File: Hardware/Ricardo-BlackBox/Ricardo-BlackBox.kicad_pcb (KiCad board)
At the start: 4 copper layers, 80.3 x 54.1 mm, 87 parts, among them IC1 XTSD08GLGEAG, IC2 CP2102N-A02-GQFN24, J1 RBUS, J2 USB_C_Receptacle_USB2.0, U1 ESP32-S3, U2 SN65HVD230, U3 LM66200DRLR, U4 MAX77827AEFD+T, U5 SC4215, Y1 40MHz±10ppm

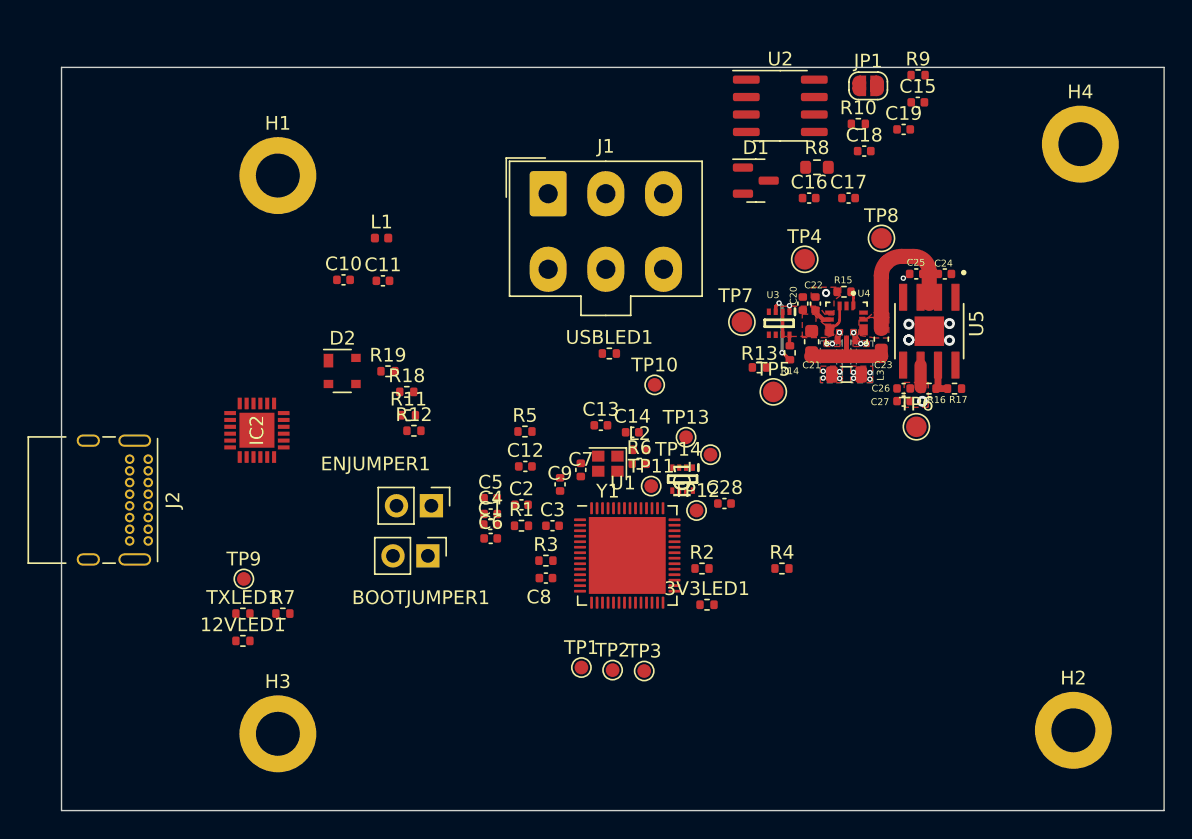
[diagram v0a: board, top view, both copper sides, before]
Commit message: Initial hardware update
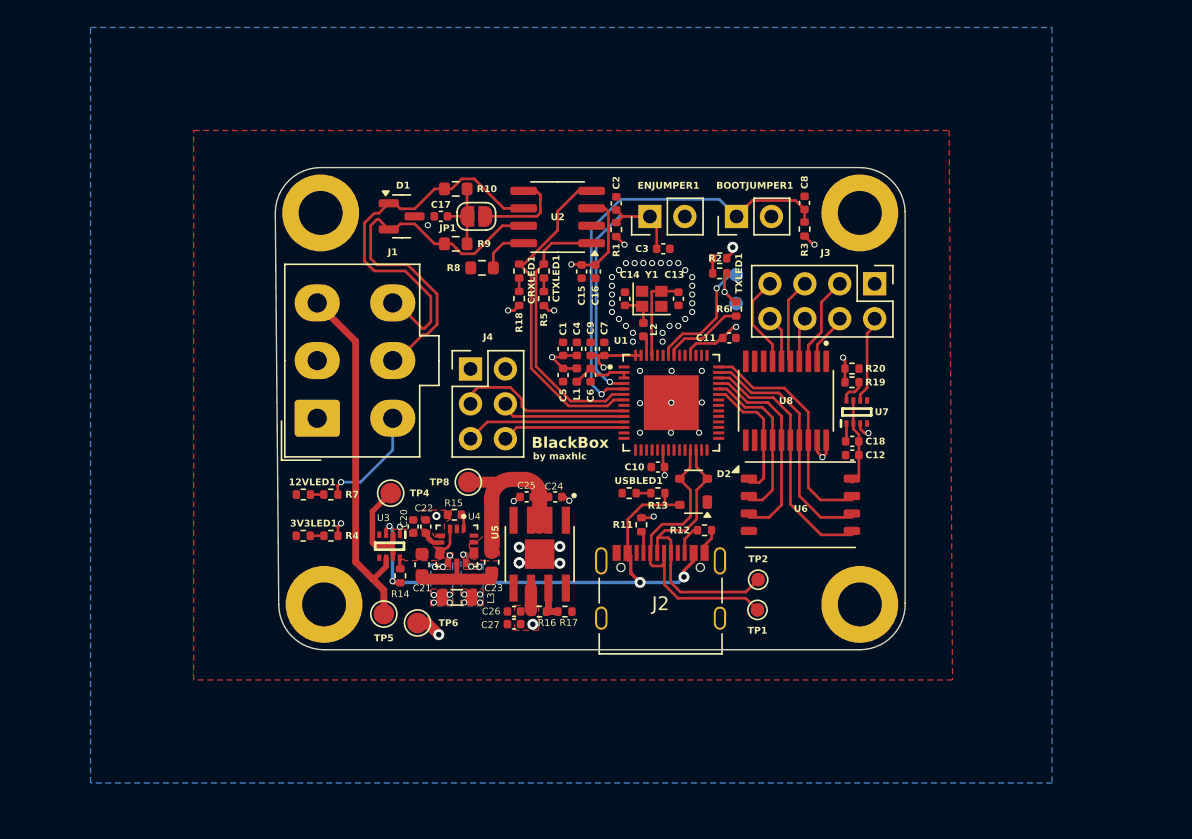
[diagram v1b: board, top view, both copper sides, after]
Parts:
- removed C19: 220pF, Capacitor_SMD:C_0402_1005Metric
- removed C28: 10uF, Capacitor_SMD:C_0402_1005Metric
- removed IC1: XTSD08GLGEAG, iclr:SOTFL50P160X60-8N
- removed IC2: CP2102N-A02-GQFN24, iclr:QFN50P400X400X80-25N
- removed TP11, TP12, TP13, TP14, TP3: TestPoint, TestPoint:TestPoint_Pad_D1.0mm
- removed TP7: TestPoint, TestPoint:TestPoint_Pad_D1.5mm
- added CRXLED1: ORANGE_LED, Resistor_SMD:R_0402_1005Metric, F.Cu at (97.1, 53.3)
- added CTXLED1: GREEN_LED, Resistor_SMD:R_0402_1005Metric, F.Cu at (98.9, 53.3)
- added J3: Conn_02x04_Odd_Even, Connector_PinHeader_2.54mm:PinHeader_2x04_P2.54mm_Vertical, F.Cu at (123.0, 54.2)
- added J4: Conn_02x03_Odd_Even, Connector_PinHeader_2.54mm:PinHeader_2x03_P2.54mm_Vertical, F.Cu at (93.6, 60.5)
- added R20: 10K, Resistor_SMD:R_0402_1005Metric, F.Cu at (121.4, 60.4)
- added U6: XTSD08G, Package_LGA:LGA-8_8x6mm_P1.27mm, F.Cu at (117.6, 70.3)
- added U7: LM66200DRLR, iclr:SOTFL50P160X60-8N, F.Cu at (121.7, 63.6)
- added U8: SN74CBTLV3245APWR, SN74CBTLV3245APWR:SOP65P640X120-20N, F.Cu at (116.5, 62.8)
- 12VLED1: value 12V_LED -> RED_LED
- 3V3LED1: value 3V3LED -> BLUE_LED
- C12: value 4.2pF -> 10uF
- C13, C14: value C -> 11pF
- C17: value 0.1uF -> 47nF
- C18: value 220pF -> 0.1uF
- J2: footprint Connector_USB:USB_C_Receptacle_GCT_USB4085 -> Connector_USB:USB_C_Receptacle_Palconn_UTC16-G
- R10, R9: footprint Resistor_SMD:R_0402_1005Metric -> Resistor_SMD:R_0603_1608Metric
- R13: value 470 -> 5.1k
- R18: value 22.1k -> 1k
- R19: value 47.5k -> 10K
- R5: value 47.5 -> 1k
- R6: value 499 -> 499R
- TP10, TP9: moved to B.Cu
- TXLED1: value TX_LED -> GREEN_LED
- U1: footprint Package_DFN_QFN:QFN-56-1EP_7x7mm_P0.4mm_EP5.6x5.6mm -> iclr:QFN40P700X700X90-57N
- U5: value SC4215 -> SC4215ASTRT
- USBLED1: value USB_LED -> WHITE_LED
- Y1: value 40MHz±10ppm -> R940000171
- moved H4 64.4 mm to (82.9, 77.6)
- moved H3 43.4 mm to (121.9, 77.6)
- moved TXLED1 42.6 mm to (111.7, 53.5), turned to 180 degrees
- moved TP9 41.1 mm to (112.9, 55.7), turned to 180 degrees
- moved H2 40.7 mm to (121.9, 49.1)
- moved TP6 39.0 mm to (89.7, 78.9)
- moved J2 38.5 mm to (107.4, 76.3), turned to 0 degrees
- moved R9 35.8 mm to (92.5, 51.3)
- moved TP8 34.9 mm to (93.4, 68.7)
- moved TP4 34.6 mm to (87.8, 69.5)
- moved R19 33.8 mm to (121.4, 61.4), turned to 180 degrees
- moved BOOTJUMPER1 33.4 mm to (113.0, 49.4), turned to 90 degrees
- moved C8 33.2 mm to (117.9, 48.4), turned to 90 degrees
- moved R4 32.9 mm to (83.4, 72.6)
- moved C21 32.7 mm to (90.1, 74.7)
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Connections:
- C12 pad 1: Net-(C12-Pad1) -> /NAND_3V3
- C12 pad 2: Net-(C12-Pad2) -> GND
- C18 pad 1: GND -> /NAND_3V3
- C18 pad 2: /CAN+ -> GND
- D2 pad 2: Net-(D2-Pad2) -> /Data+
- D2 pad 3: Net-(D2-Pad3) -> /Data-
- D2 pad 4: Net-(D2-Pad4) -> VBUS
- J2 pad A4: Net-(D2-Pad2) -> VBUS
- J2 pad A6: Net-(D2-Pad3) -> /Data+
- J2 pad A7: Net-(D2-Pad4) -> /Data-
- J2 pad A9: Net-(D2-Pad2) -> VBUS
- J2 pad B4: Net-(D2-Pad2) -> VBUS
- J2 pad B6: Net-(D2-Pad3) -> /Data+
- J2 pad B7: Net-(D2-Pad4) -> /Data-
- J2 pad B9: Net-(D2-Pad2) -> VBUS
- R18 pad 1: Net-(D2-Pad2) -> +3V3
- R18 pad 2: Net-(IC2-Pad8) -> Net-(CRXLED1-A)
- R19 pad 1: Net-(IC2-Pad8) -> Net-(U7-ST)
- R19 pad 2: GND -> +3V3
- R5 pad 1: GND -> +3V3
- R5 pad 2: Net-(C12-Pad1) -> Net-(CTXLED1-A)
- R6 pad 1: /RXD -> /TXD
- U1 pad 1: Net-(C12-Pad2) -> unconnected-(U1-LNA_IN/RF-Pad1)
- U1 pad 10: unconnected-(U1-Pad10) -> /GPIO_5
- U1 pad 11: unconnected-(U1-Pad11) -> /GPIO_6
- U1 pad 12: unconnected-(U1-Pad12) -> /GPIO_7
- U1 pad 37: unconnected-(U1-Pad37) -> /NAND_SD2
- U1 pad 38: unconnected-(U1-Pad38) -> /NAND_SD3
- U1 pad 39: unconnected-(U1-Pad39) -> /NAND_CLK
- U1 pad 40: /NAND_CS -> /NAND_CMD
- U1 pad 41: /CLK -> /NAND_SD0
- U1 pad 42: /MISO -> /NAND_SD1
- U1 pad 43: /MOSI -> unconnected-(U1-GPIO38-Pad43)
- U1 pad 50: /TXD -> /RXD
- U1 pad 6: unconnected-(U1-Pad6) -> /CAN_TX
- U1 pad 7: unconnected-(U1-Pad7) -> /CAN_RX
- U1 pad 9: unconnected-(U1-Pad9) -> /GPIO_4
- U5 pad 5: (no net) -> unconnected-(U5-NC-Pad5)
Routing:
- net +3V3: track 1.61 -> 37.6 mm, vias 1 -> 16
- net VBUS: track 5.27 -> 39.7 mm, vias 2 -> 4
- net /BOOT: track 0.00 -> 32.8 mm, vias 0 -> 1
- net /CAN+: track 0.00 -> 30.0 mm
- net /CAN-: track 0.00 -> 29.8 mm
- net RBUS_uC_V: track 0.00 -> 26.3 mm
- net /CAN_RX: track 0.00 -> 24.6 mm
- net /Data-: track 0.00 -> 22.9 mm
- net /CHIP_PU: track 0.00 -> 22.4 mm, vias 0 -> 1
- net /Data+: track 0.00 -> 21.5 mm
- net /CAN_TX: track 0.00 -> 20.0 mm
- net /NAND_CMD: track 0.00 -> 18.3 mm
- net /NAND_SD0: track 0.00 -> 17.6 mm
- net /NAND_SD1: track 0.00 -> 17.0 mm
- net /NAND_CLK: track 0.00 -> 14.7 mm
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- added copper zone on In2.Cu, net +3V3
- added copper zone on B.Cu, net GND
- added copper zone on In1.Cu, net GND
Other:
- board size 80.3 x 54.1 mm -> 45.8 x 35.1 mm
- board text added: "BlackBox"
- board text added: "by maxhlc"
